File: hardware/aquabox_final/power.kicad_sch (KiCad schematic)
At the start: 0 parts

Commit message: Atualização
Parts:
- added J2: AC 220V, symbol Connector:Screw_Terminal_01x04
- added PS1: MC00100, MC00100:CONV_MC00100, symbol MC00100:MC00100
- added RV1: MOV-14D471K, symbol Device:Varistor
- added U1: HLK-10M05, Converter_ACDC:Converter_ACDC_Hi-Link_HLK-10Mxx, symbol Converter_ACDC:HLK-10M05
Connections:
- new net: J2.1 (Pin_1), J2.2 (Pin_2), RV1.1, U1.1 (AC/L)
- new net: J2.3 (Pin_3), J2.4 (Pin_4), RV1.2, U1.2 (AC/N)
- new net: PS1.IN-, U1.3 (-Vout)
- new net +3.3V: PS1.OUT+
- new net +5V: PS1.IN+, U1.4 (+Vout)
- new net GND: PS1.MH1 (MOUTING), PS1.MH2 (MOUTING), PS1.OUT-
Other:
- note added: "AC_L_IN"
- note added: "AC_L_OUT"
- note added: "AC_N_IN"
- note added: "AC_N_OUT"

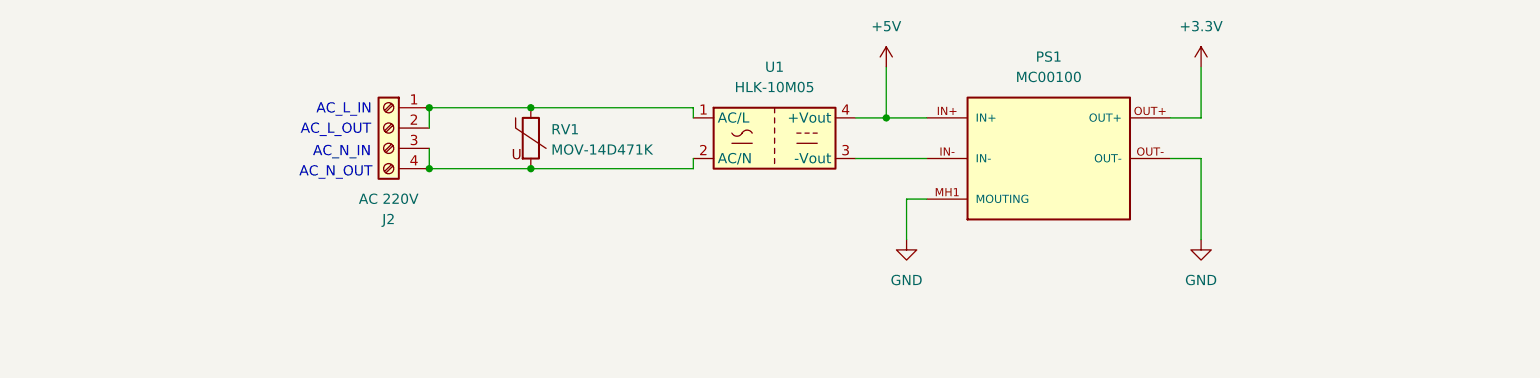
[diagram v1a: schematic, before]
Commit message: Desenvolvimento da fonte de alimentação.
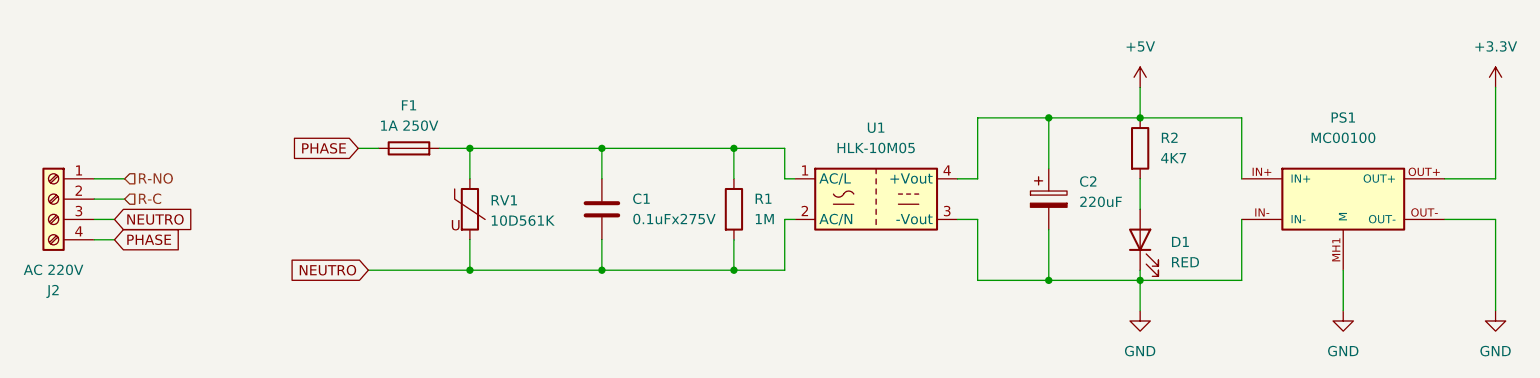
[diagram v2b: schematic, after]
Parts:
- added C1: 0.1uFx275V, symbol Device:C
- added C2: 220uF, symbol Device:C_Polarized
- added D1: RED, symbol Device:LED
- added F1: 1A 250V, symbol Device:Fuse
- added R1: 1M, symbol Device:R
- added R2: 4K7, symbol Device:R
- RV1: value MOV-14D471K -> 10D561K
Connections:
- net +5V: now also C2.1, R2.1
- net GND: now also PS1.IN-, U1.3 (-Vout), C2.2, D1.1 (K); no longer PS1.MH2 (MOUTING)
- net at RV1.1, U1.1 (AC/L): now also C1.1, F1.2, R1.1; no longer J2.1 (Pin_1), J2.2 (Pin_2)
- net NEUTRO: now reaches J2.3 (Pin_3), RV1.2, U1.2 (AC/N)
- net NEUTRO: now also C1.2, R1.2; no longer J2.4 (Pin_4)
- new net: D1.2 (A), R2.2
- new net PHASE: F1.1, J2.4 (Pin_4)
- new net R-C: J2.2 (Pin_2)
- new net R-NO: J2.1 (Pin_1)
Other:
- note removed: "AC_L_IN"
- note removed: "AC_L_OUT"
- note removed: "AC_N_IN"
- note removed: "AC_N_OUT"
- moved on the sheet: J2, PS1, RV1, U1

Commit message: Atualização
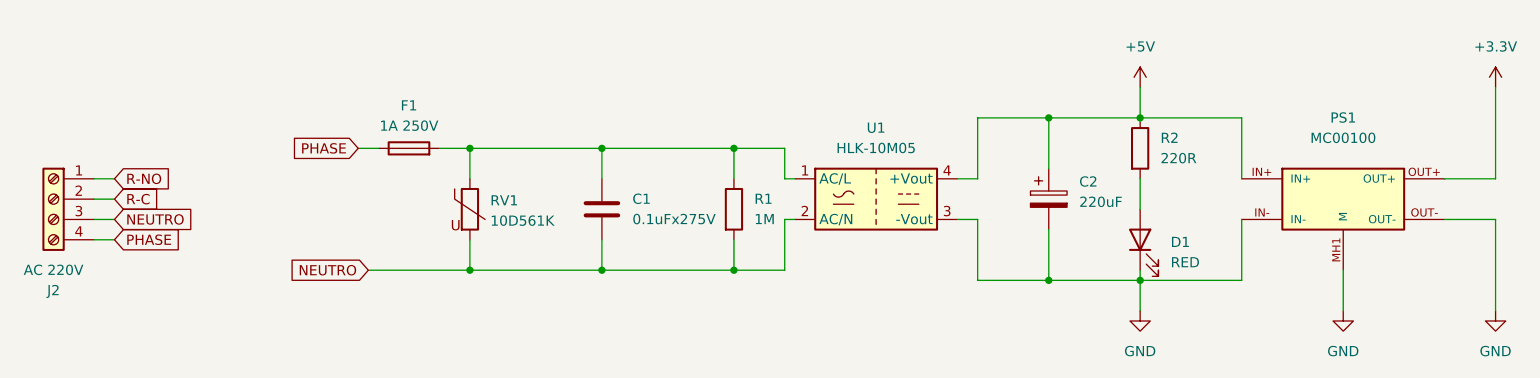
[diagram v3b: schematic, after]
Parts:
- R2: value 4K7 -> 220R
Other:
- company: (none) -> INVENCTUS - Soluções Tecnológicas
- title: (none) -> Power
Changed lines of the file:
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@@
 	(generator_version "10.0")
 	(paper "A4")
+	(title_block
+		(title "Power")
+		(date "2026-06-02")
+		(rev "1.0.0")
+		(company "INVENCTUS - Soluções Tecnológicas")
+		(comment 1 "Eng. José Adriano")
+	)
 	(junction
 		(at 190.5 86.36)
@@
 	(wire
 		(pts
-			(xy 59.69 93.98) (xy 63.5 93.98)
-		)
-		(stroke
-			(width 0)
-			(type default)
-		)
-	)
-	(wire
-		(pts
 			(xy 123.19 101.6) (xy 123.19 105.41)
 		)
@@
 	(wire
 		(pts
+			(xy 59.69 96.52) (xy 62.23 96.52)
+		)
+		(stroke
+			(width 0)
+			(type default)
+		)
+	)
+	(wire
+		(pts
 			(xy 234.95 99.06) (xy 234.95 110.49)
 		)
@@
 	(wire
 		(pts
+			(xy 59.69 93.98) (xy 62.23 93.98)
+		)
+		(stroke
+			(width 0)
+			(type default)
+		)
+	)
+	(wire
+		(pts
 			(xy 123.19 90.17) (xy 123.19 93.98)
 		)
@@
 	(wire
 		(pts
-			(xy 59.69 96.52) (xy 63.5 96.52)
-		)
-		(stroke
-			(width 0)
-			(type default)
-		)
-	)
-	(wire
-		(pts
 			(xy 190.5 93.98) (xy 190.5 97.79)
 		)
@@
 			(width 0)
 			(type default)
+		)
+	)
+	(global_label "R-C"
+		(shape input)
+		(at 62.23 96.52 0)
+		(fields_autoplaced yes)
+		(effects
+			(font
+				(size 1.27 1.27)
+			)
+			(justify left)
+		)
+		(property "Intersheetrefs" "${INTERSHEET_REFS}"
+			(at 69.3276 96.52 0)
+			(hide yes)
+			(show_name no)
+			(do_not_autoplace no)
+			(effects
+				(font
+					(size 1.27 1.27)
+				)
+				(justify left)
+			)
 		)
 	)
@@
 		)
 	)
-	(hierarchical_label "R-C"
+	(global_label "R-NO"
 		(shape input)
-		(at 63.5 96.52 0)
+		(at 62.23 93.98 0)
+		(fields_autoplaced yes)
 		(effects
 			(font
@@
 			(justify left)
 		)
-	)
-	(hierarchical_label "R-NO"
-		(shape input)
-		(at 63.5 93.98 0)
-		(effects
-			(font
-				(size 1.27 1.27)
-			)
-			(justify left)
+		(property "Intersheetrefs" "${INTERSHEET_REFS}"
+			(at 70.7186 93.98 0)
+			(hide yes)
+			(show_name no)
+			(do_not_autoplace no)
+			(effects
+				(font
+					(size 1.27 1.27)
+				)
+				(justify left)
+			)
 		)
 	)
@@
 			)
 		)
-		(property "Value" "4K7"
+		(property "Value" "220R"
 			(at 193.04 91.4399 0)
 			(show_name no)
